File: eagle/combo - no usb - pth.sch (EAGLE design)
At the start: 27 parts, among them U2 ATMEGA328P_PDIP

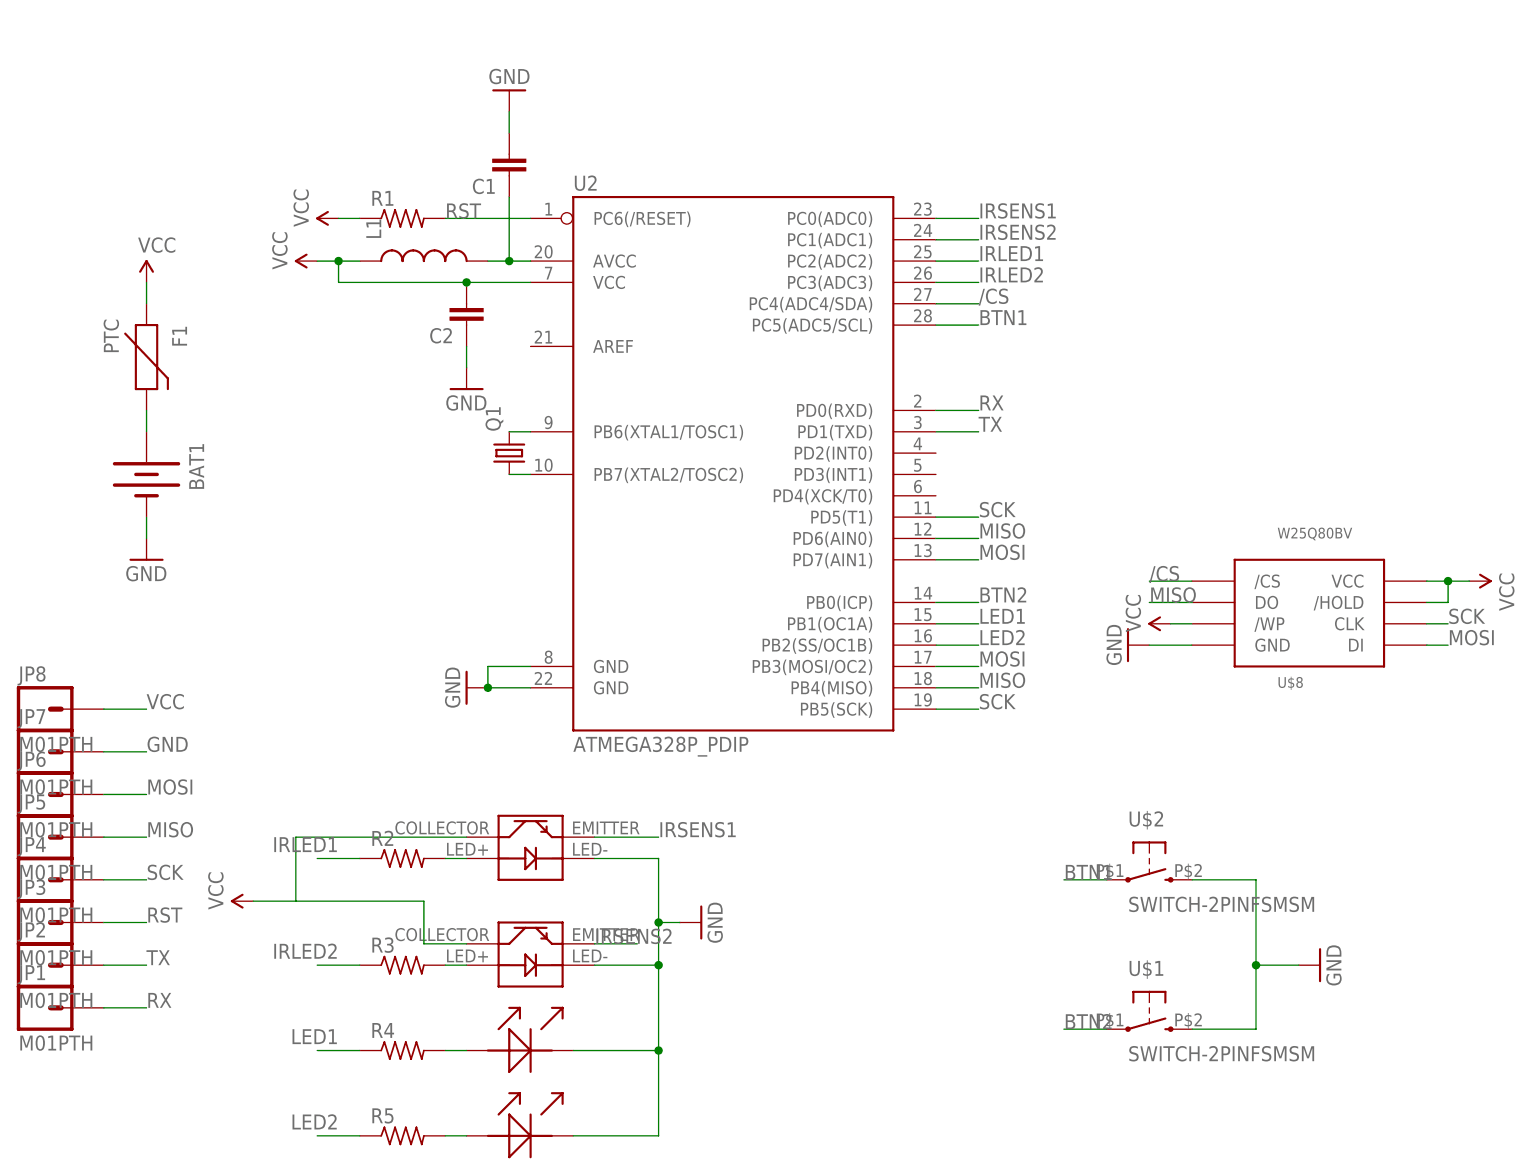
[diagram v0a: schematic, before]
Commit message: Progress routing board
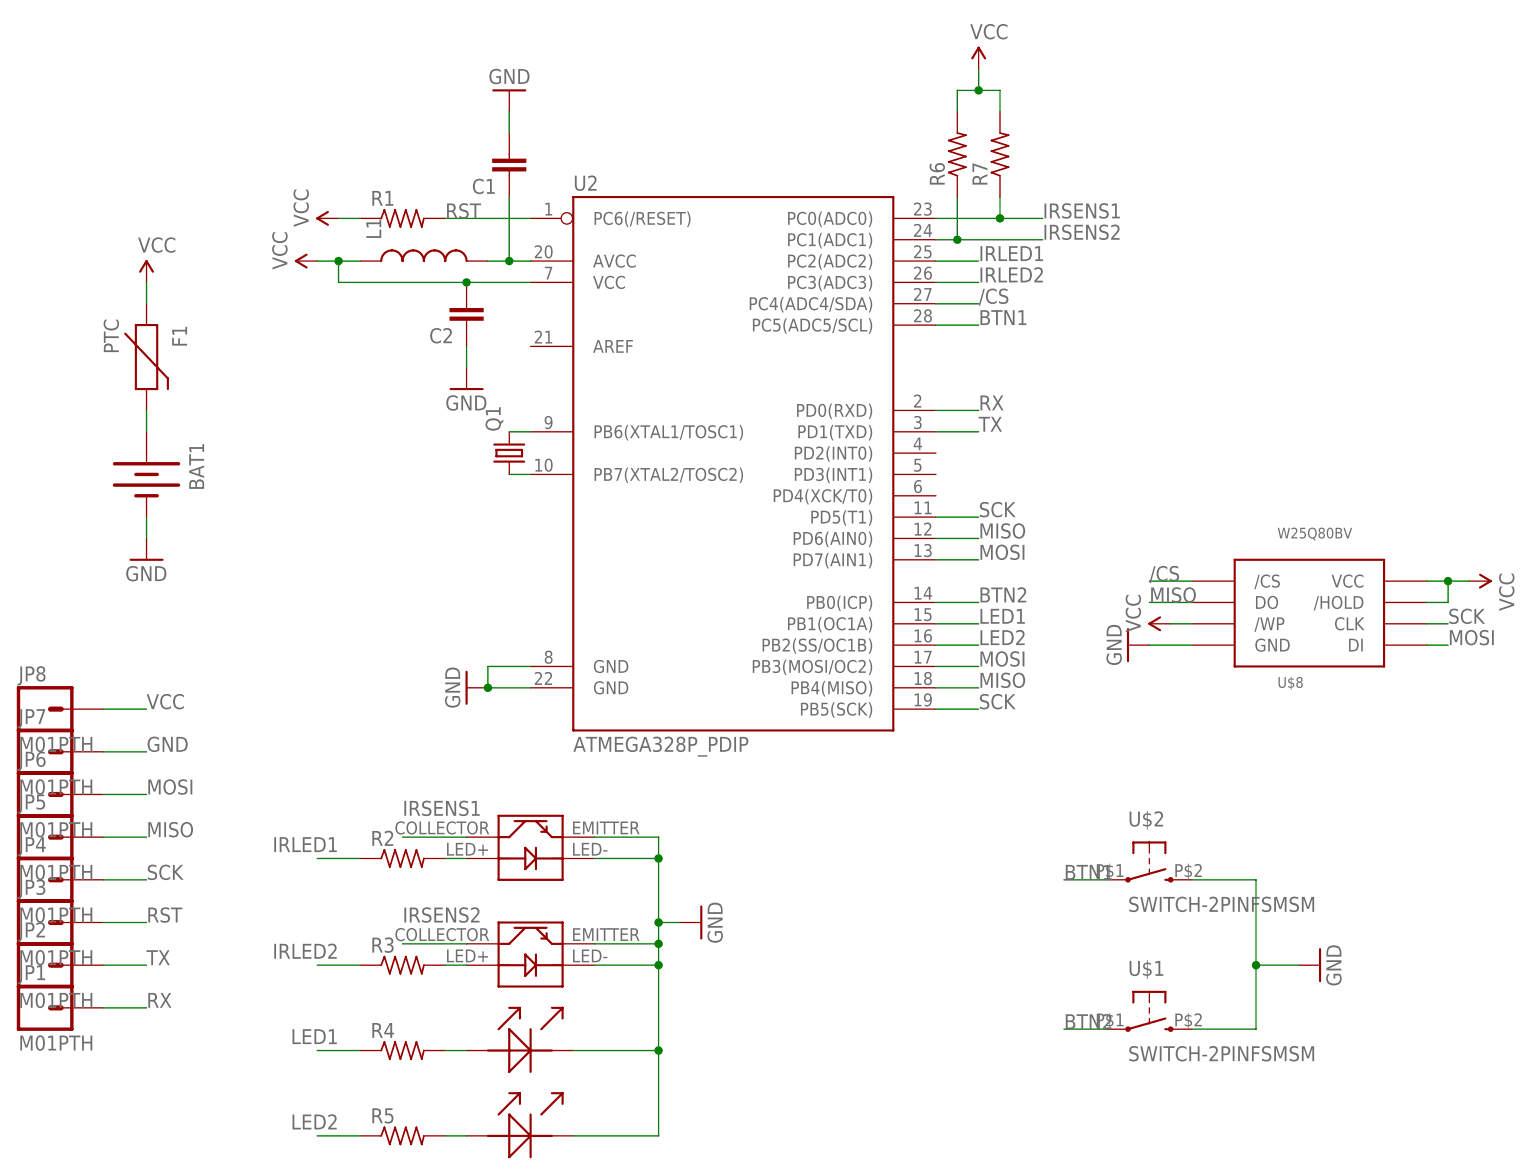
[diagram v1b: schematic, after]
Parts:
- added R6, R7: (no value), rcl:R-US_M0805
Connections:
- net GND: now also U$3.EMITTER, U$4.EMITTER
- net IRSENS1: now also R7.1, U$3.COLLECTOR; no longer U$3.EMITTER
- net IRSENS2: now also R6.1, U$4.COLLECTOR; no longer U$4.EMITTER
- net VCC: now also R6.2, R7.2; no longer U$3.COLLECTOR, U$4.COLLECTOR
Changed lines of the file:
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@@
 <part name="GND7" library="SparkFun-Aesthetics" deviceset="GND" device=""/>
 <part name="GND8" library="SparkFun-Aesthetics" deviceset="GND" device=""/>
-<part name="SUPPLY8" library="SparkFun-Aesthetics" deviceset="VCC" device=""/>
 <part name="U2" library="SparkFun-DigitalIC" deviceset="ATMEGA328P_PDIP" device=""/>
 <part name="Q1" library="crystal" deviceset="CRYSTAL" device="TC26V"/>
+<part name="R6" library="rcl" deviceset="R-US_" device="M0805"/>
+<part name="R7" library="rcl" deviceset="R-US_" device="M0805"/>
+<part name="SUPPLY3" library="SparkFun-Aesthetics" deviceset="VCC" device=""/>
 </parts>
 <sheets>
@@
 <instance part="GND7" gate="1" x="68.58" y="58.42"/>
 <instance part="GND8" gate="1" x="96.52" y="-5.08" rot="R90"/>
-<instance part="SUPPLY8" gate="1" x="43.18" y="-2.54" rot="R90"/>
 <instance part="U2" gate="G$1" x="99.06" y="53.34"/>
 <instance part="Q1" gate="G$1" x="73.66" y="50.8" rot="R90"/>
+<instance part="R6" gate="G$1" x="127" y="86.36" rot="R90"/>
+<instance part="R7" gate="G$1" x="132.08" y="86.36" rot="R90"/>
+<instance part="SUPPLY3" gate="1" x="129.54" y="96.52"/>
 </instances>
 <busses>
@@
 <pinref part="U$4" gate="G$1" pin="LED-"/>
 <wire x1="83.82" y1="-10.16" x2="91.44" y2="-10.16" width="0.1524" layer="91"/>
-<wire x1="91.44" y1="-10.16" x2="91.44" y2="-5.08" width="0.1524" layer="91"/>
+<wire x1="91.44" y1="-10.16" x2="91.44" y2="-7.62" width="0.1524" layer="91"/>
 <junction x="91.44" y="-5.08"/>
 <pinref part="GND8" gate="1" pin="GND"/>
 <pinref part="U$5" gate="G$1" pin="-"/>
+<wire x1="91.44" y1="-7.62" x2="91.44" y2="-5.08" width="0.1524" layer="91"/>
 <wire x1="81.28" y1="-20.32" x2="91.44" y2="-20.32" width="0.1524" layer="91"/>
 <wire x1="91.44" y1="-20.32" x2="91.44" y2="-10.16" width="0.1524" layer="91"/>
@@
 <wire x1="91.44" y1="-30.48" x2="91.44" y2="-20.32" width="0.1524" layer="91"/>
 <junction x="91.44" y="-20.32"/>
+<pinref part="U$4" gate="G$1" pin="EMITTER"/>
+<wire x1="83.82" y1="-7.62" x2="91.44" y2="-7.62" width="0.1524" layer="91"/>
+<junction x="91.44" y="-7.62"/>
+<pinref part="U$3" gate="G$1" pin="EMITTER"/>
+<wire x1="83.82" y1="5.08" x2="91.44" y2="5.08" width="0.1524" layer="91"/>
+<wire x1="91.44" y1="5.08" x2="91.44" y2="2.54" width="0.1524" layer="91"/>
+<junction x="91.44" y="2.54"/>
 </segment>
 </net>
@@
 </segment>
 <segment>
-<pinref part="SUPPLY8" gate="1" pin="VCC"/>
-<wire x1="43.18" y1="-2.54" x2="48.26" y2="-2.54" width="0.1524" layer="91"/>
-<pinref part="U$4" gate="G$1" pin="COLLECTOR"/>
-<wire x1="48.26" y1="-2.54" x2="63.5" y2="-2.54" width="0.1524" layer="91"/>
-<wire x1="63.5" y1="-7.62" x2="68.58" y2="-7.62" width="0.1524" layer="91"/>
-<wire x1="63.5" y1="-2.54" x2="63.5" y2="-7.62" width="0.1524" layer="91"/>
-<wire x1="48.26" y1="-2.54" x2="48.26" y2="5.08" width="0.1524" layer="91"/>
-<pinref part="U$3" gate="G$1" pin="COLLECTOR"/>
-<wire x1="48.26" y1="5.08" x2="68.58" y2="5.08" width="0.1524" layer="91"/>
+<pinref part="R6" gate="G$1" pin="2"/>
+<wire x1="127" y1="91.44" x2="127" y2="93.98" width="0.1524" layer="91"/>
+<pinref part="R7" gate="G$1" pin="2"/>
+<wire x1="132.08" y1="91.44" x2="132.08" y2="93.98" width="0.1524" layer="91"/>
+<wire x1="132.08" y1="93.98" x2="129.54" y2="93.98" width="0.1524" layer="91"/>
+<pinref part="SUPPLY3" gate="1" pin="VCC"/>
+<wire x1="129.54" y1="93.98" x2="127" y2="93.98" width="0.1524" layer="91"/>
+<wire x1="129.54" y1="93.98" x2="129.54" y2="96.52" width="0.1524" layer="91"/>
+<junction x="129.54" y="93.98"/>
 </segment>
 </net>
@@
 <net name="IRSENS1" class="0">
 <segment>
-<wire x1="124.46" y1="78.74" x2="129.54" y2="78.74" width="0.1524" layer="91"/>
-<label x="129.54" y="78.74" size="1.778" layer="95"/>
+<wire x1="124.46" y1="78.74" x2="132.08" y2="78.74" width="0.1524" layer="91"/>
+<label x="137.16" y="78.74" size="1.778" layer="95"/>
 <pinref part="U2" gate="G$1" pin="PC0(ADC0)"/>
-</segment>
-<segment>
-<pinref part="U$3" gate="G$1" pin="EMITTER"/>
-<wire x1="83.82" y1="5.08" x2="91.44" y2="5.08" width="0.1524" layer="91"/>
-<label x="91.44" y="5.08" size="1.778" layer="95"/>
+<wire x1="132.08" y1="78.74" x2="137.16" y2="78.74" width="0.1524" layer="91"/>
+<wire x1="132.08" y1="78.74" x2="132.08" y2="81.28" width="0.1524" layer="91"/>
+<junction x="132.08" y="78.74"/>
+<pinref part="R7" gate="G$1" pin="1"/>
+</segment>
+<segment>
+<pinref part="U$3" gate="G$1" pin="COLLECTOR"/>
+<wire x1="60.96" y1="5.08" x2="68.58" y2="5.08" width="0.1524" layer="91"/>
+<label x="60.96" y="7.62" size="1.778" layer="95"/>
 </segment>
 </net>
 <net name="IRSENS2" class="0">
 <segment>
-<wire x1="124.46" y1="76.2" x2="129.54" y2="76.2" width="0.1524" layer="91"/>
-<label x="129.54" y="76.2" size="1.778" layer="95"/>
+<wire x1="124.46" y1="76.2" x2="127" y2="76.2" width="0.1524" layer="91"/>
+<label x="137.16" y="76.2" size="1.778" layer="95"/>
 <pinref part="U2" gate="G$1" pin="PC1(ADC1)"/>
-</segment>
-<segment>
-<pinref part="U$4" gate="G$1" pin="EMITTER"/>
-<wire x1="83.82" y1="-7.62" x2="88.9" y2="-7.62" width="0.1524" layer="91"/>
-<label x="83.82" y="-7.62" size="1.778" layer="95"/>
-</segment>
-</net>
+<wire x1="127" y1="76.2" x2="137.16" y2="76.2" width="0.1524" layer="91"/>
+<wire x1="127" y1="76.2" x2="127" y2="81.28" width="0.1524" layer="91"/>
+<junction x="127" y="76.2"/>
+<pinref part="R6" gate="G$1" pin="1"/>
+</segment>
+<segment>
+<pinref part="U$4" gate="G$1" pin="COLLECTOR"/>
+<wire x1="60.96" y1="-7.62" x2="68.58" y2="-7.62" width="0.1524" layer="91"/>
+<label x="60.96" y="-5.08" size="1.778" layer="95"/>
+</segment>
+</net>
